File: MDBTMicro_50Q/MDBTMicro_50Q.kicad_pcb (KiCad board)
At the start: 2 copper layers, 33 x 17.8 mm, 41 parts, among them J1 ProMicro Pinout, J2 USB_C_Receptacle_USB2.0, Q1 AO3407, Q2 AO3407, U1 XC6220B331MR-G, U2 MDBT50Q-x1MV2, U3 TP4057, X1 32.768kHz

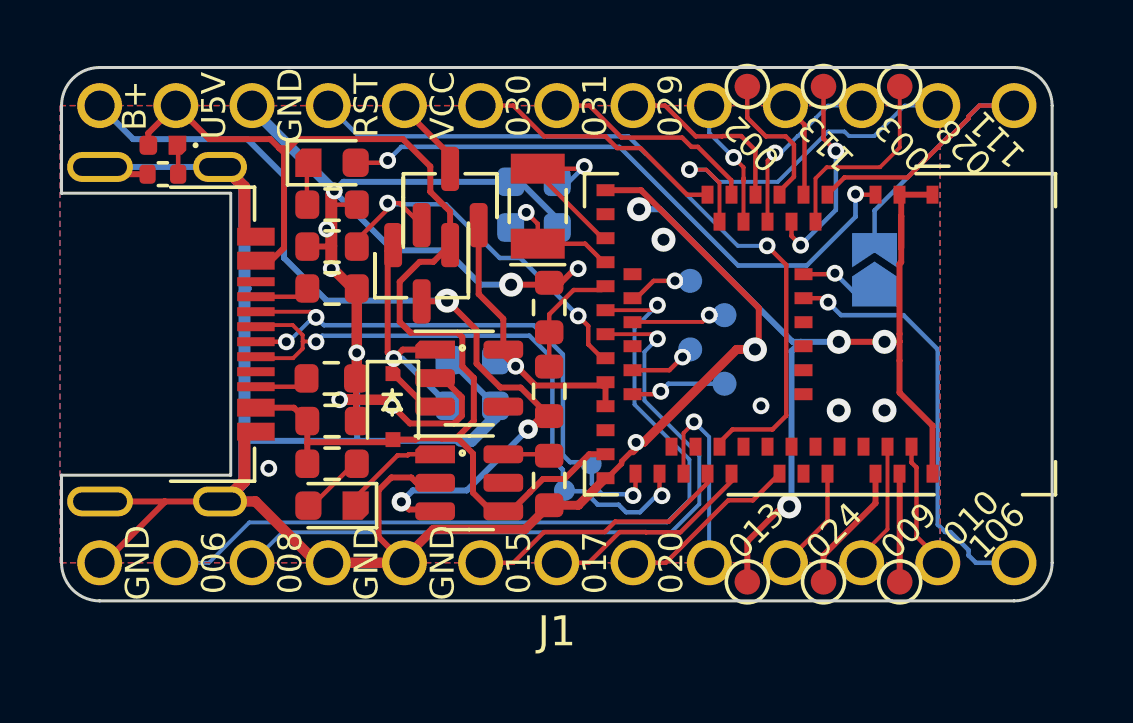
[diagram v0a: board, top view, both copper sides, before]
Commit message: Update v1.4
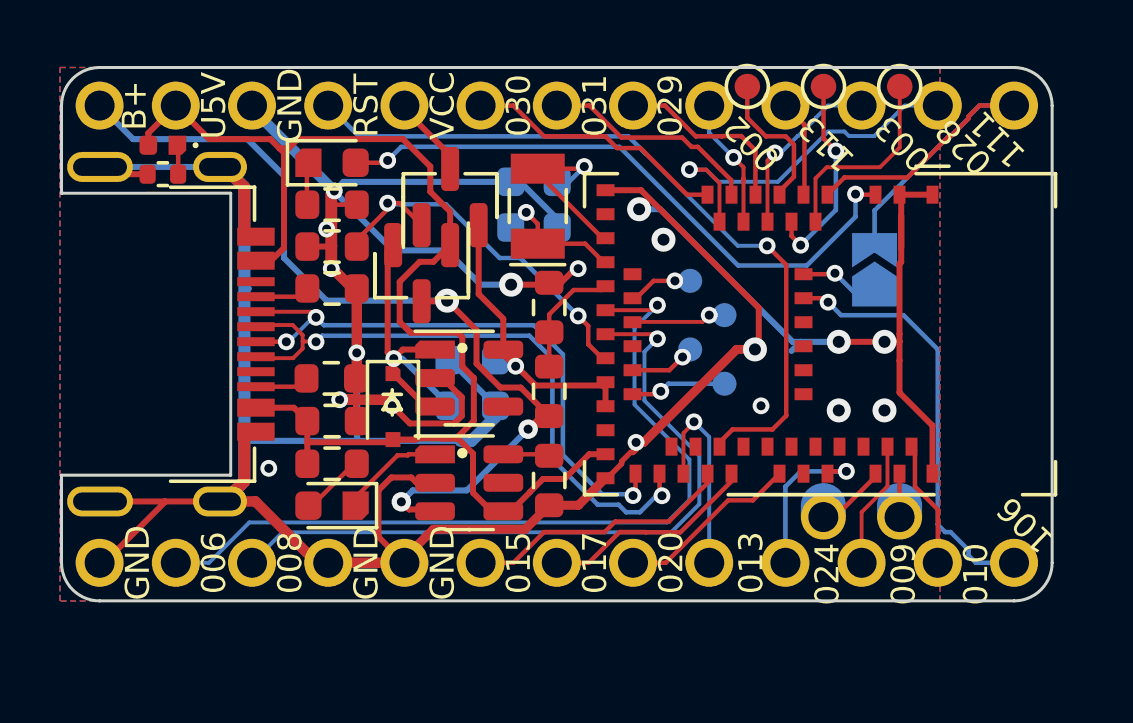
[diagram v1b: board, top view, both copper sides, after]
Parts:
- removed ? (x2): , 
- removed REF** (x2): TestPoint_Pad_D1.0mm, TestPoint:TestPoint_Pad_D1.0mm
- removed TP10: SWCLK, TestPoint:TestPoint_Pad_D1.0mm
- removed TP8: GND, TestPoint:TestPoint_Pad_D1.0mm
- removed TP9: SWDIO, TestPoint:TestPoint_Pad_D1.0mm
- added J3: Conn_01x02, Connector_PinHeader_2.54mm:PinHeader_1x02_P2.54mm_Vertical, F.Cu at (76.1, 55.5)
- added J4: Conn_01x13, Connector_PinHeader_2.54mm:PinHeader_1x13_P2.54mm_Vertical, B.Cu at (51.9, 41.8)
- J1: value ProMicro Pinout -> Conn_01x13; footprint MDBTMicro_library:ProMicro board pinout -> Connector_PinHeader_2.54mm:PinHeader_1x13_P2.54mm_Vertical; moved to B.Cu
- moved J1 17.3 mm to (51.9, 57.0), turned to -90 degrees
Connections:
- J1 pad 1: /P0.06 -> GND
- J1 pad 10: /P0.09 -> /P0.24
- J1 pad 11: /P0.10 -> /P0.09
- J1 pad 12: /P1.06 -> /P0.10
- J1 pad 13: VBUS -> /P1.06
- J1 pad 2: /P0.08 -> /P0.06
- J1 pad 3: GND -> /P0.08
- J1 pad 5: /P0.15 -> GND
- J1 pad 6: /P0.17 -> /P0.15
- J1 pad 7: /P0.20 -> /P0.17
- J1 pad 8: /P0.13 -> /P0.20
- J1 pad 9: /P0.24 -> /P0.13
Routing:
- net GND: track 150.5 -> 142.1 mm, vias 19 -> 18
- net SWCLK: track 3.61 -> 1.45 mm
- net SWDIO: track 4.32 -> 2.39 mm
- net /P0.24: track 3.55 -> 5.44 mm, vias 0 -> 1
- net USB_D-: track 21.3 -> 20.6 mm
- net USB_D+: track 22.4 -> 21.7 mm
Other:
- board text added: "v${REVISION}"
- board text removed: "10"
- board text removed: "14"
- board text removed: "15"
- board text removed: "16"
- board text removed: "2"
- board text removed: "3"
- board text removed: "4"
- board text removed: "5"
- board text removed: "6"
- board text removed: "7"
- board text removed: "8"
- board text removed: "9"
- board text removed: "A0"
- board text removed: "A1"
- board text removed: "A2"
- board text removed: "A3"
- board text removed: "B +"
- board text removed: "G"
- board text removed: "Rx0"
- board text removed: "Tx1"
- board text removed: "v1.3"
